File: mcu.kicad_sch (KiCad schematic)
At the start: 8 parts, among them J20 LOLIN-S3 (L), J21 LOLIN-S3 (R), J22 ESP32-S3-DEVKITC-1 (L), J23 ESP32-S3-DEVKITC-1 (R), J24 LOLIN-S3-MINI (L), J25 LOLIN-S3-MINI (R), J26 LOLIN-S2-MINI (L), J27 LOLIN-S2-MINI (R)

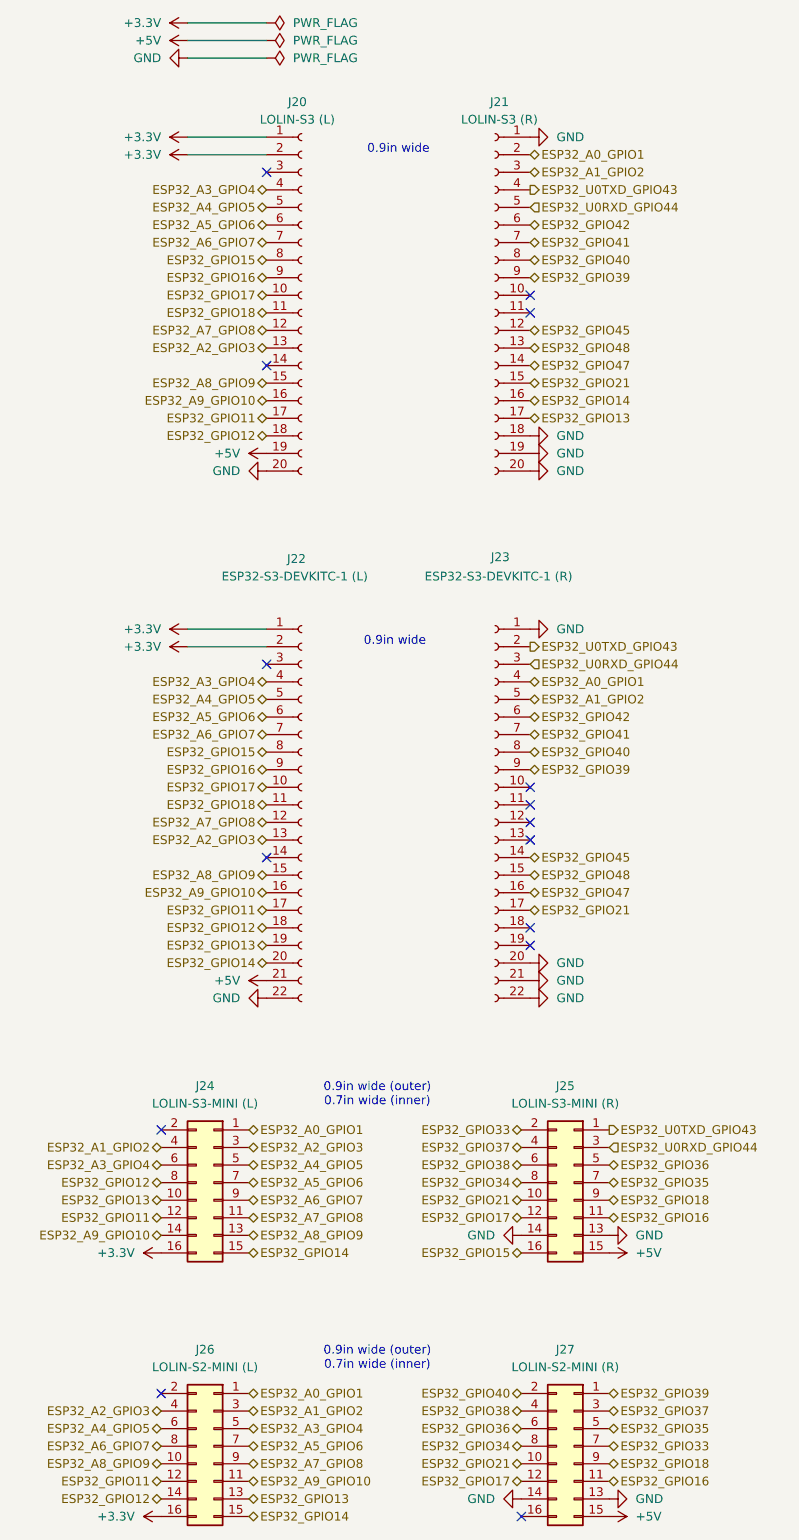
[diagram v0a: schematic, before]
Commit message: Render PCB
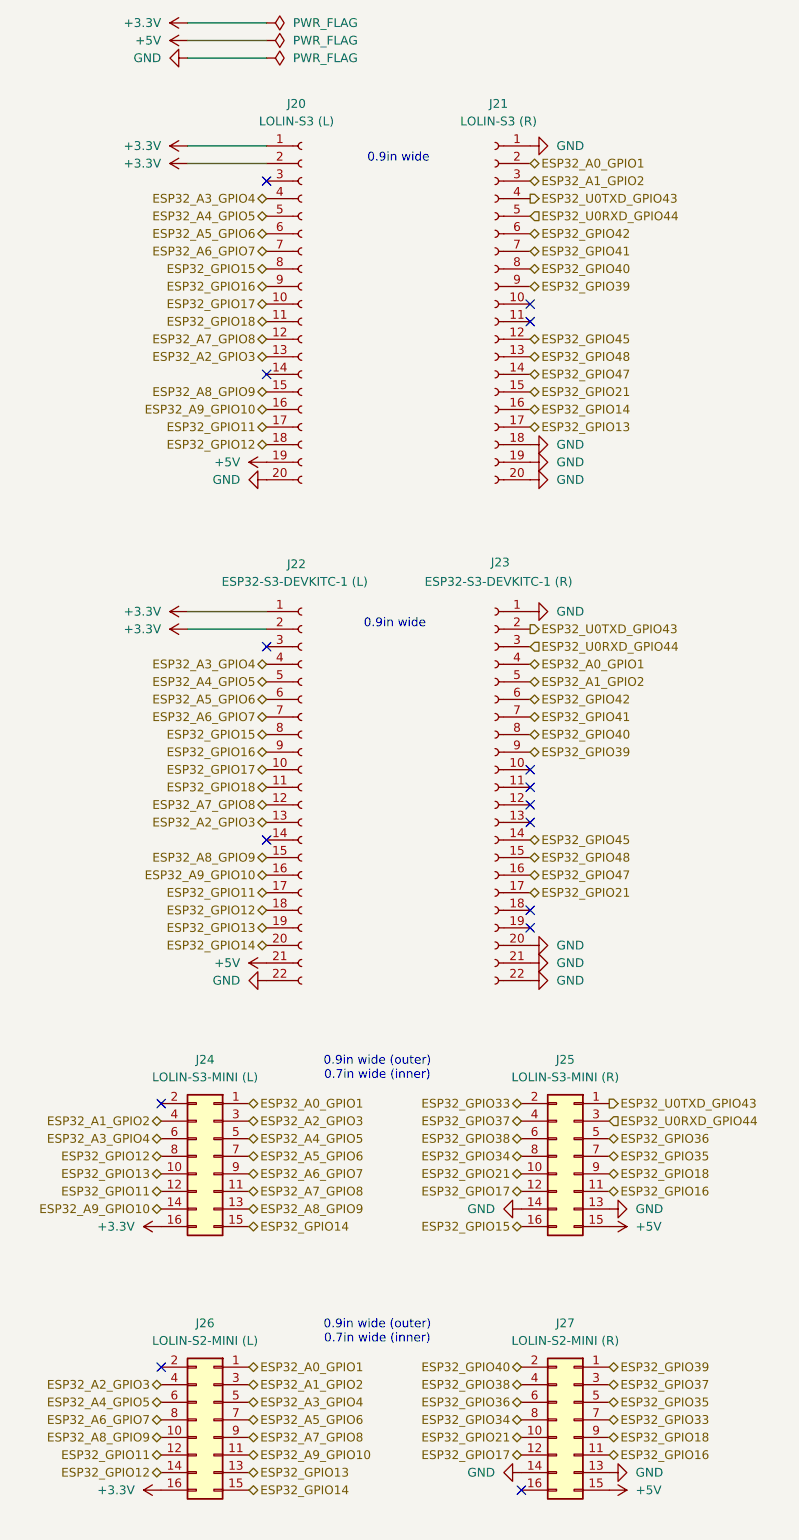
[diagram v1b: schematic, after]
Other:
- moved on the sheet: J20, J21, J22, J23, J24, J25, J26, J27
